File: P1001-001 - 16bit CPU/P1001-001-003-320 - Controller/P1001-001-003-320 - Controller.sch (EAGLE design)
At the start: 154 parts, among them IC1 74LS138D, IC10 74ALS00D, IC21 74LS138D, IC22 74LS138D, IC23 74LS138D, IC27 MEGA8535-A, IC3 74LS138D, IC4 74LS138D, IC5 74LS138D, J1 22-27-2041-04

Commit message: Controller done?
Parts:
- removed ADD_HIGH, ADD_LOW, ADD_MID, BA_HIGH, BA_LOW, BB_HIGH, BB_LOW, BC_HIGH, BC_LOW: 74ABT164D, 74xx-us:74ABT164D
- removed JP4: (no value), jumper:JP3Q
- removed R12, R13, R14: (no value), rcl:R-US_M0805
- removed READ_WRITE: (no value), jumper:JP2E
- removed SW_PROD_1, SW_PROD_2, SW_PROD_3, SW_PROD_4, SW_PROD_5: 74LS157D, 74xx-us:74LS157D
- added SV2: (no value), con-harting-ml:ML6
- BANKA, BANKB, BANKC: value SST39VF1602-70-4I-EKE -> (none); device 16bit:SST39VF1602-70-4I-EKE -> con-harting-ml:ML16
- JP3: device jumper:JP6Q -> pinhead:PINHD-1X20
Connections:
- removed net ADDR_BUS0: BANKA.A0, BANKB.A0, BANKC.A0, SW_PROD_1A.4Y
- removed net ADDR_BUS1: BANKA.A1, BANKB.A1, BANKC.A1, SW_PROD_1A.3Y
- removed net ADDR_BUS10: BANKA.A10, BANKB.A10, BANKC.A10, SW_PROD_3A.2Y
- removed net ADDR_BUS11: BANKA.A11, BANKB.A11, BANKC.A11, SW_PROD_3A.1Y
- removed net ADDR_BUS12: BANKA.A12, BANKB.A12, BANKC.A12, SW_PROD_4A.1Y
- removed net ADDR_BUS13: BANKA.A13, BANKB.A13, BANKC.A13, SW_PROD_4A.2Y
- removed net ADDR_BUS14: BANKA.A14, BANKB.A14, BANKC.A14, SW_PROD_4A.3Y
- removed net ADDR_BUS15: BANKA.A15, BANKB.A15, BANKC.A15, SW_PROD_4A.4Y
- removed net ADDR_BUS16: BANKA.A16, BANKB.A16, BANKC.A16, SW_PROD_5A.1Y
- removed net ADDR_BUS17: BANKA.A17, BANKB.A17, BANKC.A17, SW_PROD_5A.2Y
- removed net ADDR_BUS18: BANKA.A18, BANKB.A18, BANKC.A18, SW_PROD_5A.3Y
- removed net ADDR_BUS19: BANKA.A19, BANKB.A19, BANKC.A19, SW_PROD_5A.4Y
- removed net ADDR_BUS2: BANKA.A2, BANKB.A2, BANKC.A2, SW_PROD_1A.2Y
- removed net ADDR_BUS3: BANKA.A3, BANKB.A3, BANKC.A3, SW_PROD_1A.1Y
- removed net ADDR_BUS4: BANKA.A4, BANKB.A4, BANKC.A4, SW_PROD_2A.4Y
- removed net ADDR_BUS5: BANKA.A5, BANKB.A5, BANKC.A5, SW_PROD_2A.3Y
- removed net ADDR_BUS6: BANKA.A6, BANKB.A6, BANKC.A6, SW_PROD_2A.2Y
- removed net ADDR_BUS7: BANKA.A7, BANKB.A7, BANKC.A7, SW_PROD_2A.1Y
- removed net ADDR_BUS8: BANKA.A8, BANKB.A8, BANKC.A8, SW_PROD_3A.4Y
- removed net ADDR_BUS9: BANKA.A9, BANKB.A9, BANKC.A9, SW_PROD_3A.3Y
- removed net ADDR_SHIFT: ADD_LOWA.A, ADD_LOWA.B, JP3.5
- removed net BANKA_PROG: BANKA.!WE, JP4.5, R12.1
- removed net BANKB_PROG: BANKB.!WE, JP4.3, R13.1
- removed net BANKC_PROG: BANKC.!WE, JP4.1, R14.1
- removed net DATAA_SHIFT: BA_LOWA.A, BA_LOWA.B, JP3.6
- removed net DATAB_SHIFT: BB_LOWA.A, BB_LOWA.B, JP3.4
- removed net DATAC_SHIFT: BC_LOWA.A, BC_LOWA.B, JP3.3
- removed net DATA_ADDR_CLOCK: BA_HIGHA.CLK, BA_LOWA.CLK, BB_HIGHA.CLK, BB_LOWA.CLK, BC_HIGHA.CLK, BC_LOWA.CLK, JP3.7
- removed net N$37: BANKA.VSS, BANKA.VSS2, BANKB.VSS, BANKB.VSS2, BANKC.VSS, BANKC.VSS2
- removed net N$42: BANKA.!OE, BANKB.!OE, BANKC.!OE, READ_WRITE.2
- removed net PROGRAM: JP3.9, JP4.2, JP4.4, JP4.6
- removed net PROG_ADDR0: ADD_LOWA.QA, SW_PROD_1A.4B
- removed net PROG_ADDR1: ADD_LOWA.QB, SW_PROD_1A.3B
- removed net PROG_ADDR10: ADD_MIDA.QC, SW_PROD_3A.2B
- removed net PROG_ADDR11: ADD_MIDA.QD, SW_PROD_3A.1B
- removed net PROG_ADDR12: ADD_MIDA.QE, SW_PROD_4A.1B
- removed net PROG_ADDR13: ADD_MIDA.QF, SW_PROD_4A.2B
- removed net PROG_ADDR14: ADD_MIDA.QG, SW_PROD_4A.3B
- removed net PROG_ADDR15: ADD_HIGHA.A, ADD_HIGHA.B, ADD_MIDA.QH, SW_PROD_4A.4B
- removed net PROG_ADDR16: ADD_HIGHA.QA, SW_PROD_5A.1B
- removed net PROG_ADDR17: ADD_HIGHA.QB, SW_PROD_5A.2B
- removed net PROG_ADDR18: ADD_HIGHA.QC, SW_PROD_5A.3B
- removed net PROG_ADDR19: ADD_HIGHA.QD, SW_PROD_5A.4B
- removed net PROG_ADDR2: ADD_LOWA.QC, SW_PROD_1A.2B
- removed net PROG_ADDR3: ADD_LOWA.QD, SW_PROD_1A.1B
- removed net PROG_ADDR4: ADD_LOWA.QE, SW_PROD_2A.4B
- removed net PROG_ADDR5: ADD_LOWA.QF, SW_PROD_2A.3B
- removed net PROG_ADDR6: ADD_LOWA.QG, SW_PROD_2A.2B
- removed net PROG_ADDR7: ADD_LOWA.QH, ADD_MIDA.A, ADD_MIDA.B, SW_PROD_2A.1B
- removed net PROG_ADDR8: ADD_MIDA.QA, SW_PROD_3A.4B
- removed net PROG_ADDR9: ADD_MIDA.QB, SW_PROD_3A.3B
- removed net PROG_ADDR_CLOCK: ADD_HIGHA.CLK, ADD_LOWA.CLK, ADD_MIDA.CLK, JP3.8
- removed net PROG_CLEAR: ADD_HIGHA.CLR, ADD_LOWA.CLR, ADD_MIDA.CLR, BA_HIGHA.CLR, BA_LOWA.CLR, BB_HIGHA.CLR, BB_LOWA.CLR, BC_HIGHA.CLR, BC_LOWA.CLR, JP3.10
- removed net PROG_DIR: JP3.1, SW_PROD_1A.!A!/B, SW_PROD_2A.!A!/B, SW_PROD_3A.!A!/B, SW_PROD_4A.!A!/B, SW_PROD_5A.!A!/B
- removed net WRITE_ENABLE: BANKA.!WP, BANKB.!WP, BANKC.!WP, JP3.2
- net !CLEAR: no longer BANKA.!RST, BANKB.!RST, BANKC.!RST
- net DATAA0: now also BANKA.1; no longer BANKA.DQ0, BA_LOWA.QA
- net DATAA1: now also BANKA.2; no longer BANKA.DQ1, BA_LOWA.QB
- net DATAA10: now also BANKA.11; no longer BANKA.DQ10, BA_HIGHA.QC
- net DATAA11: now also BANKA.12; no longer BANKA.DQ11, BA_HIGHA.QD
- net DATAA12: now also BANKA.13; no longer BANKA.DQ12, BA_HIGHA.QE
- net DATAA13: now also BANKA.14; no longer BANKA.DQ13, BA_HIGHA.QF
- net DATAA14: now also BANKA.15; no longer BANKA.DQ14, BA_HIGHA.QG
- net DATAA15: now also BANKA.16; no longer BANKA.DQ15, BA_HIGHA.QH
- net DATAA2: now also BANKA.3; no longer BANKA.DQ2, BA_LOWA.QC
- net DATAA3: now also BANKA.4; no longer BANKA.DQ3, BA_LOWA.QD
- net DATAA4: now also BANKA.5; no longer BANKA.DQ4, BA_LOWA.QE
- net DATAA5: now also BANKA.6; no longer BANKA.DQ5, BA_LOWA.QF
- net DATAA6: now also BANKA.7; no longer BANKA.DQ6, BA_LOWA.QG
- net DATAA7: now also BANKA.8; no longer BANKA.DQ7, BA_HIGHA.A, BA_HIGHA.B, BA_LOWA.QH
- net DATAA8: now also BANKA.9; no longer BANKA.DQ8, BA_HIGHA.QA
- net DATAA9: now also BANKA.10; no longer BANKA.DQ9, BA_HIGHA.QB
- net DATAB0: now also BANKB.1; no longer BANKB.DQ0, BB_LOWA.QA
- net DATAB1: now also BANKB.2; no longer BANKB.DQ1, BB_LOWA.QB
- net DATAB10: now also BANKB.11; no longer BANKB.DQ10, BB_HIGHA.QC
- net DATAB11: now also BANKB.12; no longer BANKB.DQ11, BB_HIGHA.QD
- net DATAB12: now also BANKB.13; no longer BANKB.DQ12, BB_HIGHA.QE
- net DATAB13: now also BANKB.14; no longer BANKB.DQ13, BB_HIGHA.QF
- net DATAB14: now also BANKB.15; no longer BANKB.DQ14, BB_HIGHA.QG
- net DATAB15: now also BANKB.16; no longer BANKB.DQ15, BB_HIGHA.QH
- net DATAB2: now also BANKB.3; no longer BANKB.DQ2, BB_LOWA.QC
- net DATAB3: now also BANKB.4; no longer BANKB.DQ3, BB_LOWA.QD
- net DATAB4: now also BANKB.5; no longer BANKB.DQ4, BB_LOWA.QE
- net DATAB5: now also BANKB.6; no longer BANKB.DQ5, BB_LOWA.QF
- net DATAB6: now also BANKB.7; no longer BANKB.DQ6, BB_LOWA.QG
- net DATAB7: now also BANKB.8; no longer BANKB.DQ7, BB_HIGHA.A, BB_HIGHA.B, BB_LOWA.QH
- net DATAB8: now also BANKB.9; no longer BANKB.DQ8, BB_HIGHA.QA
- net DATAB9: now also BANKB.10; no longer BANKB.DQ9, BB_HIGHA.QB
- net DATAC0: now also BANKC.1; no longer BANKC.DQ0, BC_LOWA.QA
- net DATAC1: now also BANKC.2; no longer BANKC.DQ1, BC_LOWA.QB
- net DATAC10: now also BANKC.11; no longer BANKC.DQ10, BC_HIGHA.QC
- net DATAC11: now also BANKC.12; no longer BANKC.DQ11, BC_HIGHA.QD
- net DATAC12: now also BANKC.13; no longer BANKC.DQ12, BC_HIGHA.QE
- net DATAC13: now also BANKC.14; no longer BANKC.DQ13, BC_HIGHA.QF
- net DATAC14: now also BANKC.15; no longer BANKC.DQ14, BC_HIGHA.QG
- net DATAC15: now also BANKC.16; no longer BANKC.DQ15, BC_HIGHA.QH
- net DATAC2: now also BANKC.3; no longer BANKC.DQ2, BC_LOWA.QC
- net DATAC3: now also BANKC.4; no longer BANKC.DQ3, BC_LOWA.QD
- net DATAC4: now also BANKC.5; no longer BANKC.DQ4, BC_LOWA.QE
- net DATAC5: now also BANKC.6; no longer BANKC.DQ5, BC_LOWA.QF
- net DATAC6: now also BANKC.7; no longer BANKC.DQ6, BC_LOWA.QG
- net DATAC7: now also BANKC.8; no longer BANKC.DQ7, BC_HIGHA.A, BC_HIGHA.B, BC_LOWA.QH
- net DATAC8: now also BANKC.9; no longer BANKC.DQ8, BC_HIGHA.QA
- net DATAC9: now also BANKC.10; no longer BANKC.DQ9, BC_HIGHA.QB
- net GND: now also SV2.2, SV2.3; no longer BANKA.!CE, BANKA.VDD, BANKB.!CE, BANKB.VDD, BANKC.!CE, BANKC.VDD, JP3.11, READ_WRITE.3, SW_PROD_1A.G, SW_PROD_2A.G, SW_PROD_3A.G, SW_PROD_4A.G, SW_PROD_5A.G
- net IN_BUS0: now also JP3.20; no longer SW_PROD_1A.4A
- net IN_BUS1: now also JP3.10; no longer SW_PROD_1A.3A
- net IN_BUS10: now also JP3.15; no longer SW_PROD_3A.2A
- net IN_BUS11: now also JP3.5; no longer SW_PROD_3A.1A
- net IN_BUS12: now also JP3.14; no longer SW_PROD_4A.1A
- net IN_BUS13: now also JP3.4; no longer SW_PROD_4A.2A
- net IN_BUS14: now also JP3.13; no longer SW_PROD_4A.3A
- net IN_BUS15: now also JP3.3; no longer SW_PROD_4A.4A
- net IN_BUS16: now also JP3.12; no longer SW_PROD_5A.1A
- net IN_BUS17: now also JP3.2; no longer SW_PROD_5A.2A
- net IN_BUS18: now also JP3.11; no longer SW_PROD_5A.3A
- net IN_BUS19: now also JP3.1; no longer SW_PROD_5A.4A
- net IN_BUS2: now also JP3.19; no longer SW_PROD_1A.2A
- net IN_BUS3: now also JP3.9; no longer SW_PROD_1A.1A
- net IN_BUS4: now also JP3.18; no longer SW_PROD_2A.4A
- net IN_BUS5: now also JP3.8; no longer SW_PROD_2A.3A
- net IN_BUS6: now also JP3.17; no longer SW_PROD_2A.2A
- net IN_BUS7: now also JP3.7; no longer SW_PROD_2A.1A
- net IN_BUS8: now also JP3.16; no longer SW_PROD_3A.4A
- net IN_BUS9: now also JP3.6; no longer SW_PROD_3A.3A
- net VCC: now also SV2.1, SV2.4, SV2.5, SV2.6; no longer JP3.12, R12.2, R13.2, R14.2, READ_WRITE.1

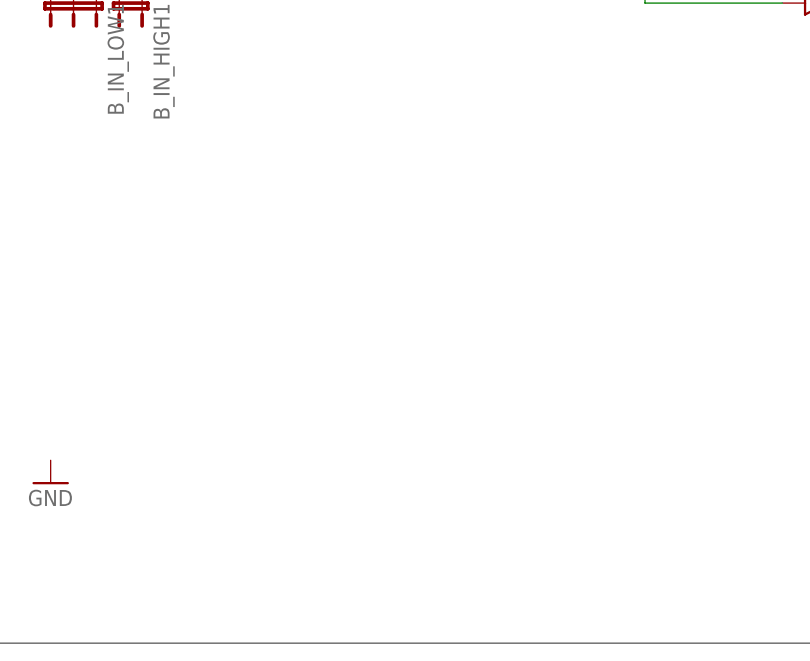
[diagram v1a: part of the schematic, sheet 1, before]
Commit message: Finished All Boards
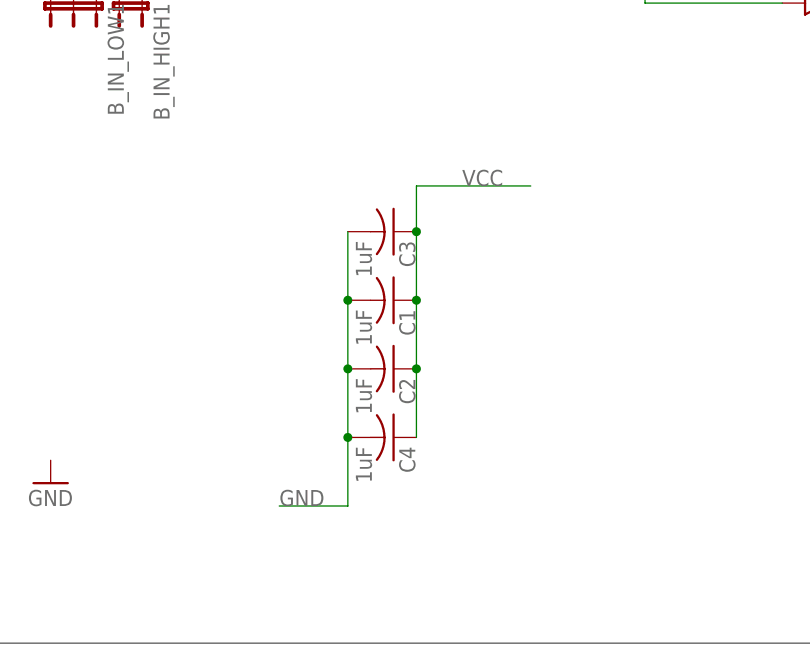
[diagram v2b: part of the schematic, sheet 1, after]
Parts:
- added C1, C2, C3, C4: 1uF, rcl:C-USC1206
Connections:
- net GND: now also C1.2, C2.2, C3.2, C4.2
- net VCC: now also C1.1, C2.1, C3.1, C4.1
